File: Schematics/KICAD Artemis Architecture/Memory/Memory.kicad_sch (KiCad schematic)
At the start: 2 parts, among them IC1 AT28C64B-15PU, IC2 AS7C164A-15PCN

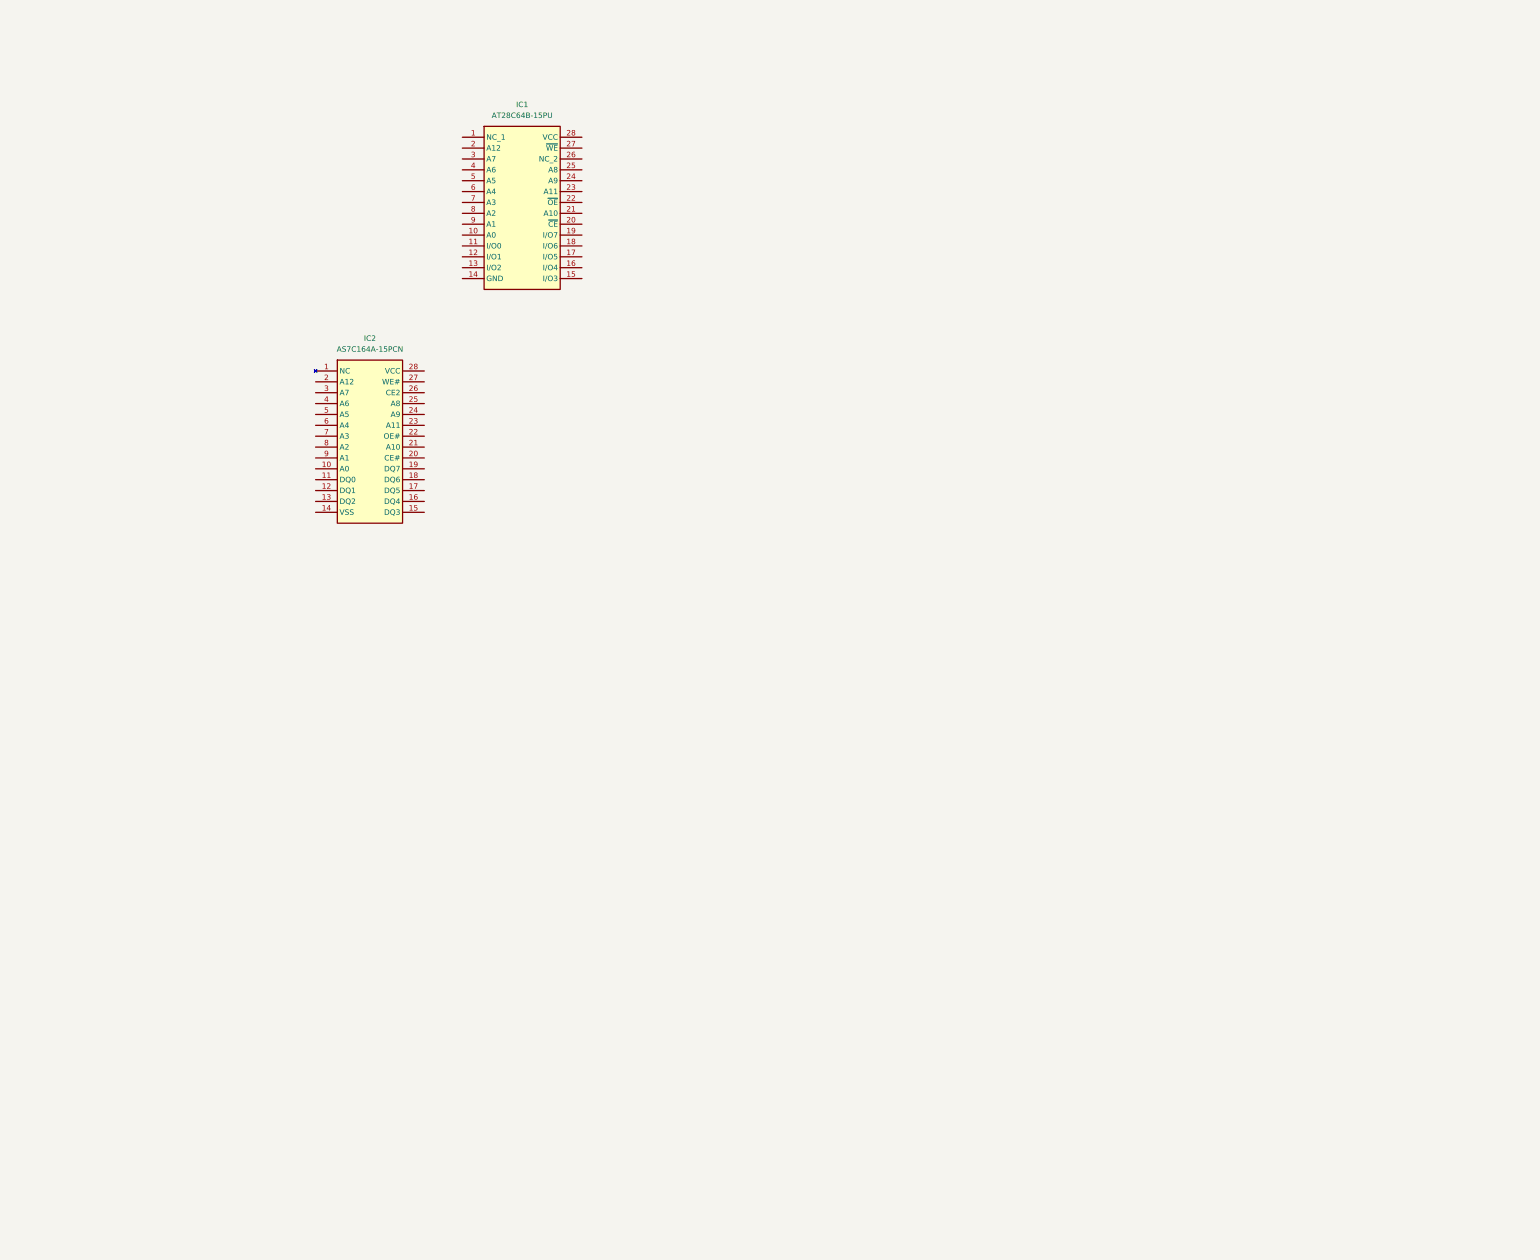
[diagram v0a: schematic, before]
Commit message: Program Memory
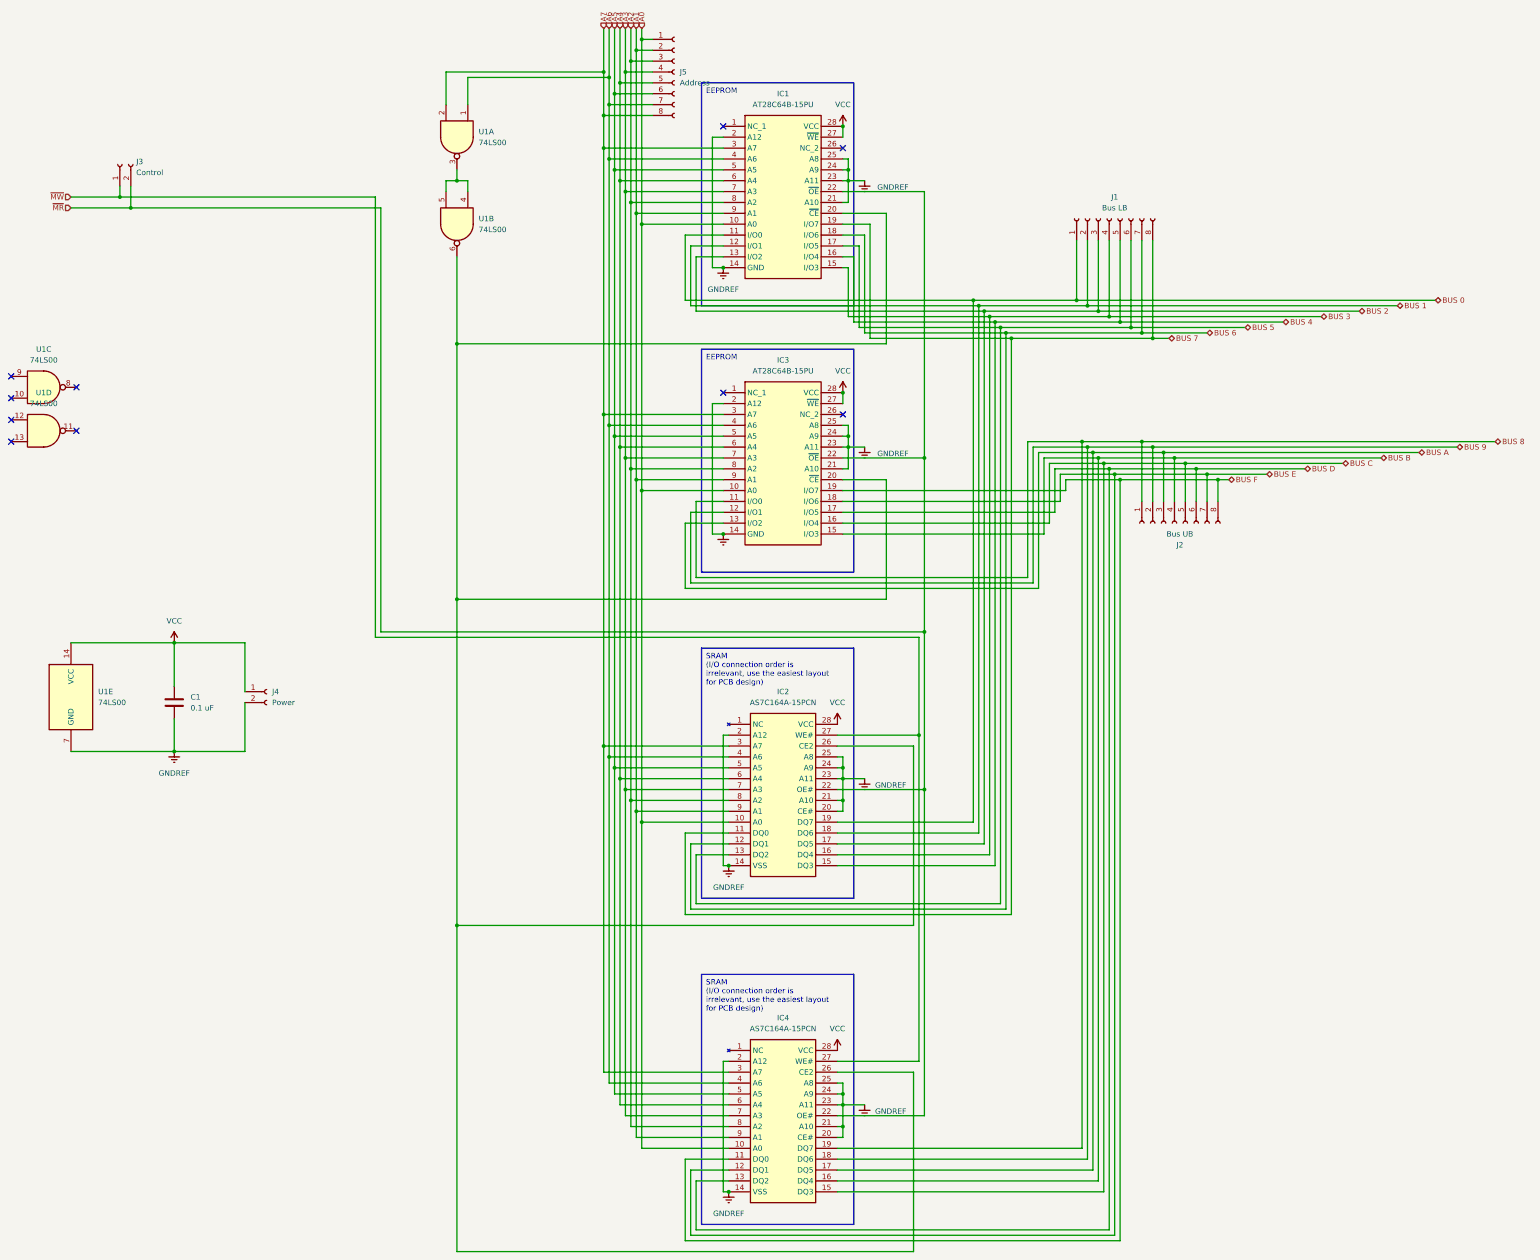
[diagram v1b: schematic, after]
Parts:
- added C1: 0.1 uF, Capacitor_SMD:C_1206_3216Metric_Pad1.33x1.80mm_HandSolder, symbol Device:C
- added IC3: AT28C64B-15PU, AT28C64B-15PU:DIP1556W56P254L3702H483Q28N, symbol AT28C64B-15PU:AT28C64B-15PU
- added IC4: AS7C164A-15PCN, AS7C164A-15PCN:DIP1524W51P254L3632H394Q28N, symbol AS7C164A-15PCN:AS7C164A-15PCN
- added J1: Bus LB, Connector_Molex:Molex_PicoBlade_53048-0810_1x08_P1.25mm_Horizontal, symbol Connector:Conn_01x08_Socket
- added J2: Bus UB, Connector_Molex:Molex_PicoBlade_53048-0810_1x08_P1.25mm_Horizontal, symbol Connector:Conn_01x08_Socket
- added J3: Control, Connector_Molex:Molex_PicoBlade_53048-0210_1x02_P1.25mm_Horizontal, symbol Connector:Conn_01x02_Socket
- added J4: Power, Connector_Molex:Molex_PicoBlade_53048-0210_1x02_P1.25mm_Horizontal, symbol Connector:Conn_01x02_Socket
- added J5: Address, Connector_Molex:Molex_PicoBlade_53048-0810_1x08_P1.25mm_Horizontal, symbol Connector:Conn_01x08_Socket
- added U1: 74LS00, Package_DIP:DIP-14_W7.62mm_Socket_LongPads, symbol 74xx:74LS00
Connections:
- net A0: now reaches IC1.10 (A0)
- net A0: now also IC2.10 (A0), IC3.10 (A0), IC4.10 (A0), J5.1 (Pin_1)
- net BUS 0: now reaches IC1.11 (I/O0)
- net BUS 0: now also IC2.19 (DQ7), J1.1 (Pin_1)
- net BUS 1: now reaches IC1.12 (I/O1)
- net BUS 1: now also IC2.18 (DQ6), J1.2 (Pin_2)
- net BUS 2: now reaches IC1.13 (I/O2)
- net BUS 2: now also IC2.17 (DQ5), J1.3 (Pin_3)
- net GNDREF: now reaches IC1.14 (GND)
- net GNDREF: now also IC1.2 (A12), IC1.21 (A10), IC1.23 (A11), IC1.24 (A9), IC1.25 (A8), IC2.14 (VSS), IC2.2 (A12), IC2.20 (CE#), IC2.21 (A10), IC2.23 (A11), IC2.24 (A9), IC2.25 (A8), C1.2, IC3.14 (GND), IC3.2 (A12), IC3.21 (A10), IC3.23 (A11), IC3.24 (A9), IC3.25 (A8), IC4.14 (VSS), IC4.2 (A12), IC4.20 (CE#), IC4.21 (A10), IC4.23 (A11), IC4.24 (A9), IC4.25 (A8), J4.2 (Pin_2), U1.7 (GND)
- net BUS 3: now reaches IC1.15 (I/O3)
- net BUS 3: now also IC2.16 (DQ4), J1.4 (Pin_4)
- net BUS 4: now reaches IC1.16 (I/O4)
- net BUS 4: now also IC2.15 (DQ3), J1.5 (Pin_5)
- net BUS 5: now reaches IC1.17 (I/O5)
- net BUS 5: now also IC2.13 (DQ2), J1.6 (Pin_6)
- net BUS 6: now reaches IC1.18 (I/O6)
- net BUS 6: now also IC2.12 (DQ1), J1.7 (Pin_7)
- net BUS 7: now reaches IC1.19 (I/O7)
- net BUS 7: now also IC2.11 (DQ0), J1.8 (Pin_8)
- net at IC1.20 (~{CE}): now also IC2.26 (CE2), IC3.20 (~{CE}), IC4.26 (CE2), U1.6
- net ~{MR}: now reaches IC1.22 (~{OE})
- net ~{MR}: now also IC2.22 (OE#), IC3.22 (~{OE}), IC4.22 (OE#), J3.2 (Pin_2)
- net VCC: now reaches IC1.27 (~{WE})
- net VCC: now also IC1.28 (VCC), IC2.28 (VCC), C1.1, IC3.27 (~{WE}), IC3.28 (VCC), IC4.28 (VCC), J4.1 (Pin_1), U1.14 (VCC)
- net A7: now reaches IC1.3 (A7)
- net A7: now also IC2.3 (A7), IC3.3 (A7), IC4.3 (A7), J5.8 (Pin_8), U1.2
- net A6: now reaches IC1.4 (A6)
- net A6: now also IC2.4 (A6), IC3.4 (A6), IC4.4 (A6), J5.7 (Pin_7), U1.1
- net A5: now reaches IC1.5 (A5)
- net A5: now also IC2.5 (A5), IC3.5 (A5), IC4.5 (A5), J5.6 (Pin_6)
- net A4: now reaches IC1.6 (A4)
- net A4: now also IC2.6 (A4), IC3.6 (A4), IC4.6 (A4), J5.5 (Pin_5)
- net A3: now reaches IC1.7 (A3)
- net A3: now also IC2.7 (A3), IC3.7 (A3), IC4.7 (A3), J5.4 (Pin_4)
- net A2: now reaches IC1.8 (A2)
- net A2: now also IC2.8 (A2), IC3.8 (A2), IC4.8 (A2), J5.3 (Pin_3)
- net A1: now reaches IC1.9 (A1)
- net A1: now also IC2.9 (A1), IC3.9 (A1), IC4.9 (A1), J5.2 (Pin_2)
- net ~{MW}: now reaches IC2.27 (WE#)
- net ~{MW}: now also IC4.27 (WE#), J3.1 (Pin_1)
- new net: U1.3, U1.4, U1.5
- new net BUS 8: IC3.11 (I/O0), IC4.19 (DQ7), J2.1 (Pin_1)
- new net BUS 9: IC3.12 (I/O1), IC4.18 (DQ6), J2.2 (Pin_2)
- new net BUS A: IC3.13 (I/O2), IC4.17 (DQ5), J2.3 (Pin_3)
- new net BUS B: IC3.15 (I/O3), IC4.16 (DQ4), J2.4 (Pin_4)
- new net BUS C: IC3.16 (I/O4), IC4.15 (DQ3), J2.5 (Pin_5)
- new net BUS D: IC3.17 (I/O5), IC4.13 (DQ2), J2.6 (Pin_6)
- new net BUS E: IC3.18 (I/O6), IC4.12 (DQ1), J2.7 (Pin_7)
- new net BUS F: IC3.19 (I/O7), IC4.11 (DQ0), J2.8 (Pin_8)
- no-connect marks 0 -> 10
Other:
- moved on the sheet: IC1, IC2

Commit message: Memory rework pt.1
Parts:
- removed J3: Control, Connector_Molex:Molex_PicoBlade_53048-0210_1x02_P1.25mm_Horizontal, symbol Connector:Conn_01x02_Socket
- removed J4: Power, Connector_Molex:Molex_PicoBlade_53048-0210_1x02_P1.25mm_Horizontal, symbol Connector:Conn_01x02_Socket
- removed J5: Address, Connector_Molex:Molex_PicoBlade_53048-0810_1x08_P1.25mm_Horizontal, symbol Connector:Conn_01x08_Socket
- added C2: 0.1 uF, Capacitor_SMD:C_1206_3216Metric_Pad1.33x1.80mm_HandSolder, symbol Device:C
- added D1, D2, D3, D4, D5, D6, D7, D8: LED, LED_SMD:LED_1206_3216Metric_Pad1.42x1.75mm_HandSolder, symbol Device:LED
- added J3: Control, Connector_Molex:Molex_PicoBlade_53048-0410_1x04_P1.25mm_Horizontal, symbol Connector:Conn_01x04_Socket
- added J4: Power, Connector_Molex:Molex_PicoBlade_53048-0410_1x04_P1.25mm_Horizontal, symbol Connector:Conn_01x04_Socket
- added R1, R2, R3, R4, R5, R6, R7, R8: 220, Resistor_SMD:R_1206_3216Metric_Pad1.30x1.75mm_HandSolder, symbol Device:R
- added U2, U4: 74LS173, Package_DIP:DIP-16_W7.62mm_Socket_LongPads, symbol 74xx:74LS173
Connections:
- net BUS 0: now also U4.11 (D3)
- net BUS 1: now also U4.12 (D2)
- net BUS 2: now also U4.13 (D1)
- net BUS 3: now also U4.14 (D0)
- net BUS 4: now also U2.11 (D3)
- net BUS 5: now also U2.12 (D2)
- net BUS 6: now also U2.13 (D1)
- net BUS 7: now also U2.14 (D0)
- net GNDREF: now also C2.2, J4.2 (Pin_2), R1.2, R2.2, R3.2, R4.2, R5.2, R6.2, R7.2, R8.2, U2.1 (Oe1), U2.2 (Oe2), U2.8 (GND), U4.1 (Oe1), U4.2 (Oe2), U4.8 (GND)
- net VCC: now also J4.1 (Pin_1), U2.16 (VCC), U4.16 (VCC)
- net A0: no longer names the net of IC1.10 (A0), IC2.10 (A0), IC3.10 (A0), IC4.10 (A0)
- net A0: now also D8.2 (A), U4.6 (Q3)
- net A1: no longer names the net of IC1.9 (A1), IC2.9 (A1), IC3.9 (A1), IC4.9 (A1)
- net A1: now also D7.2 (A), U4.5 (Q2)
- net A2: no longer names the net of IC1.8 (A2), IC2.8 (A2), IC3.8 (A2), IC4.8 (A2)
- net A2: now also D6.2 (A), U4.4 (Q1)
- net A3: no longer names the net of IC1.7 (A3), IC2.7 (A3), IC3.7 (A3), IC4.7 (A3)
- net A3: now also D5.2 (A), U4.3 (Q0)
- net A4: no longer names the net of IC1.6 (A4), IC2.6 (A4), IC3.6 (A4), IC4.6 (A4)
- net A4: now also D4.2 (A), U2.6 (Q3)
- net A5: no longer names the net of IC1.5 (A5), IC2.5 (A5), IC3.5 (A5), IC4.5 (A5)
- net A5: now also D3.2 (A), U2.5 (Q2)
- net A6: no longer names the net of IC1.4 (A6), IC2.4 (A6), IC3.4 (A6), IC4.4 (A6), U1.1
- net A6: now also D2.2 (A), U2.4 (Q1)
- net A7: no longer names the net of IC1.3 (A7), IC2.3 (A7), IC3.3 (A7), IC4.3 (A7), U1.2
- net A7: now also D1.2 (A), U2.3 (Q0)
- net ~{MR} renamed ~{MvR}
- net ~{MvR}: now also J3.3 (Pin_3)
- net ~{MW} renamed ~{MvW}
- net ~{MvW}: now also J3.2 (Pin_2)
- new net: D3.1 (K), R3.1
- new net: D5.1 (K), R5.1
- new net: D1.1 (K), R1.1
- new net: D8.1 (K), R8.1
- new net: D6.1 (K), R6.1
- new net: D7.1 (K), R7.1
- new net: D4.1 (K), R4.1
- new net: D2.1 (K), R2.1
- new net CLK: J4.3 (Pin_3), U2.7 (Cp), U4.7 (Cp)
- new net CLR: C2.1, J4.4 (Pin_4), U2.15 (Mr), U4.15 (Mr)
- new net ~{MaI}: J3.1 (Pin_1), U2.10 (E2), U2.9 (E1), U4.10 (E2), U4.9 (E1)
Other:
- moved on the sheet: C1, IC1, IC2, IC3, IC4, J1, J2, U1A, U1B, U1C, U1D, U1E
